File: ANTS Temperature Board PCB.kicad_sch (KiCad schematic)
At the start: 15 parts, among them J1 1751251, J2 1751251, J3 EBWA-02-A, J4 EBWA-02-A, J5 EBWA-02-A, J6 B2B-XH-A, Q1 IRLZ34N, Q2 IRLZ34N, U1 RASPBERRY_PI_PICO

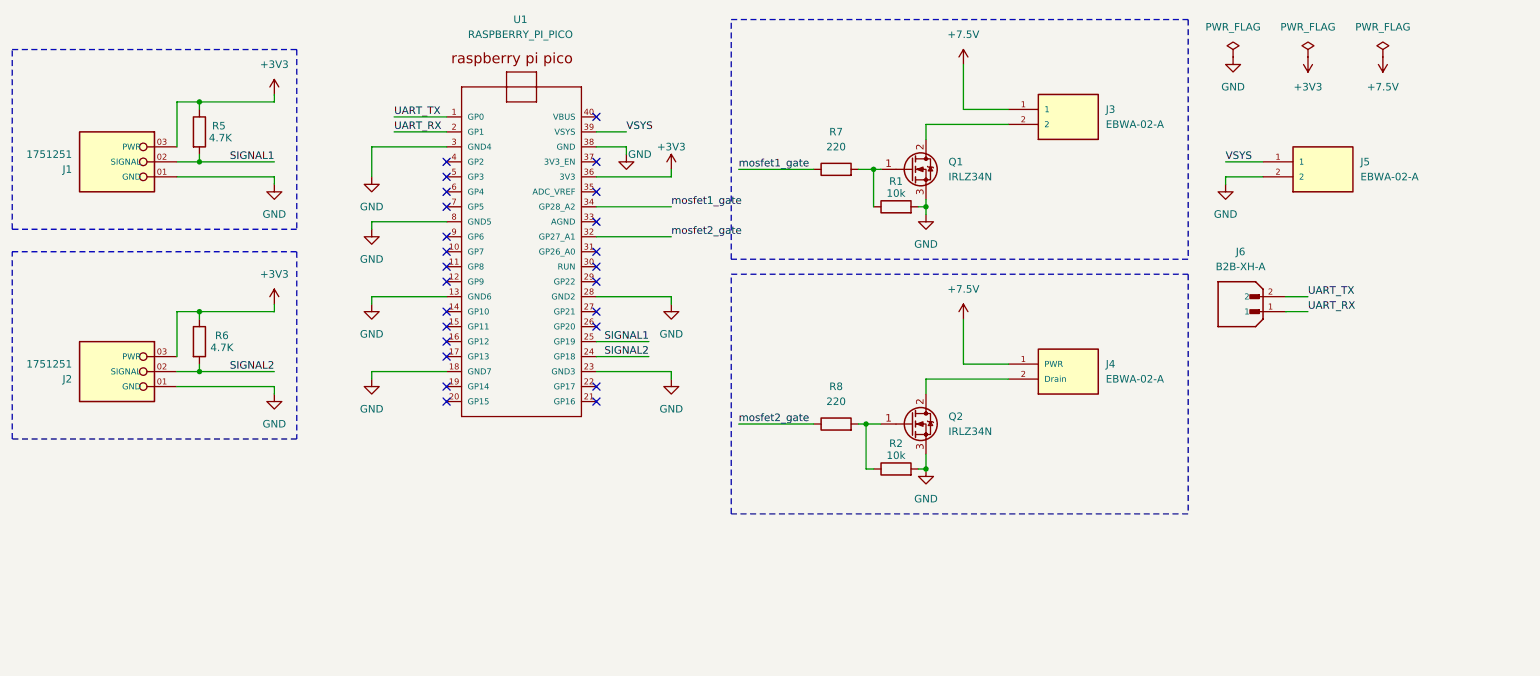
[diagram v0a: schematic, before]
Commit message: No major new changes.
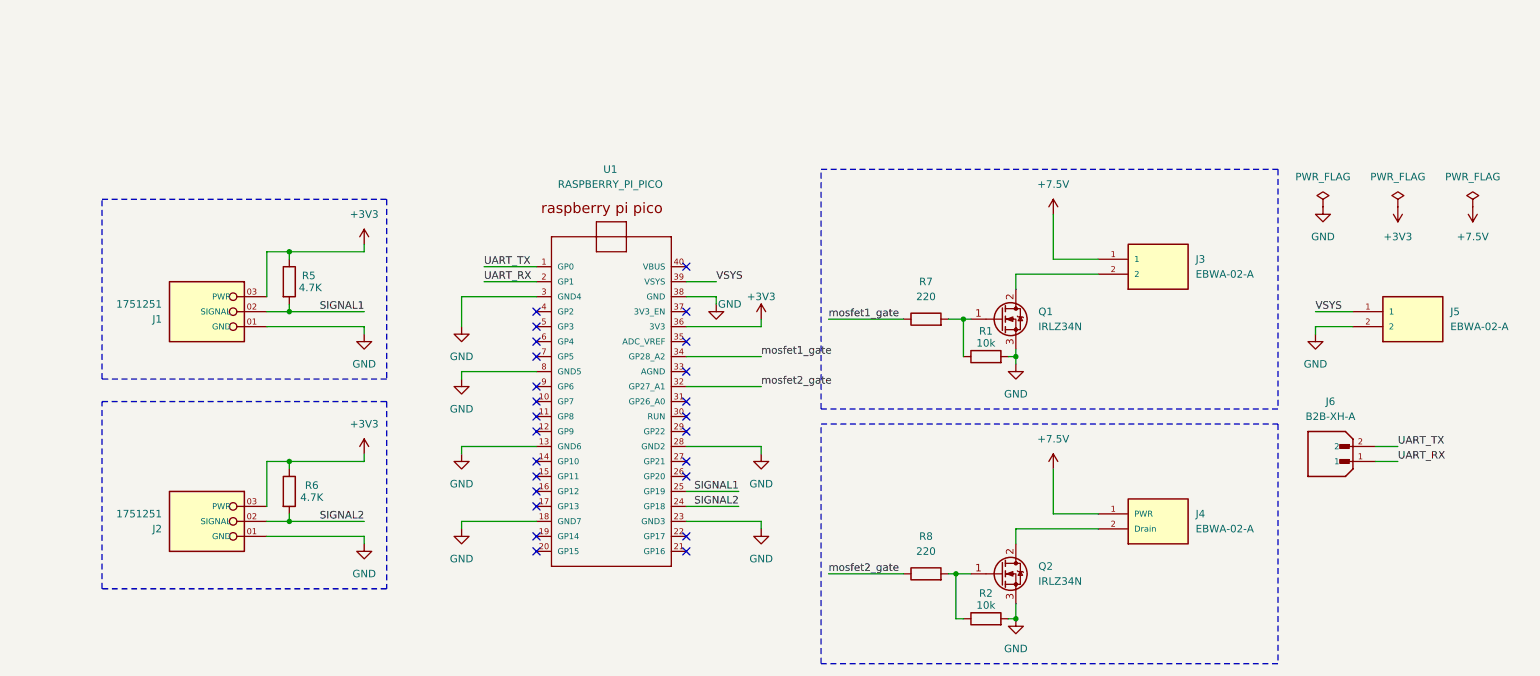
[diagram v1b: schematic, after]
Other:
- moved on the sheet: J1, J2, J3, J4, J5, J6, Q1, Q2, R1, R2, R5, R6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
